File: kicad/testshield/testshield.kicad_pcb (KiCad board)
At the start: 2 copper layers, 26.7 x 55.9 mm, 6 parts, among them J1 ISP header, J2 Raspiheader, SW1 SW_Push, U1 ATMEGA328P-PU

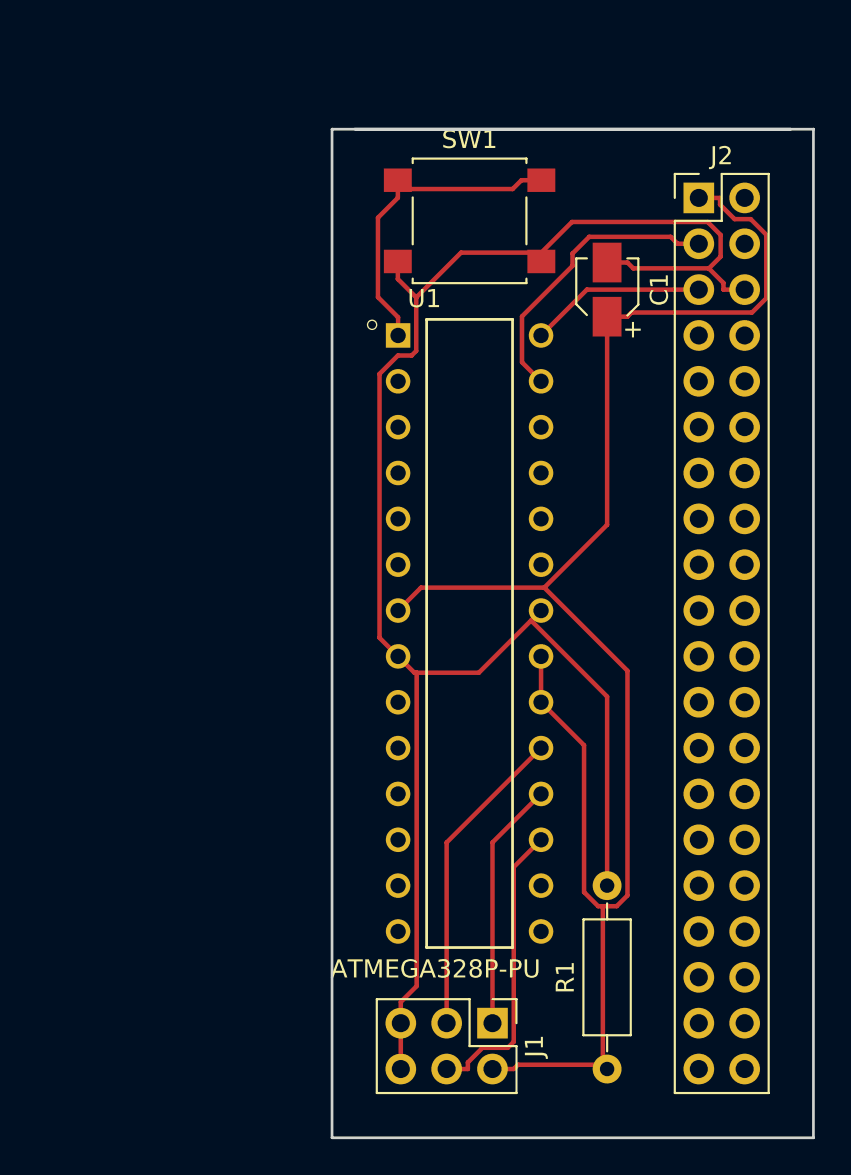
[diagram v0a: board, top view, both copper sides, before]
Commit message: update
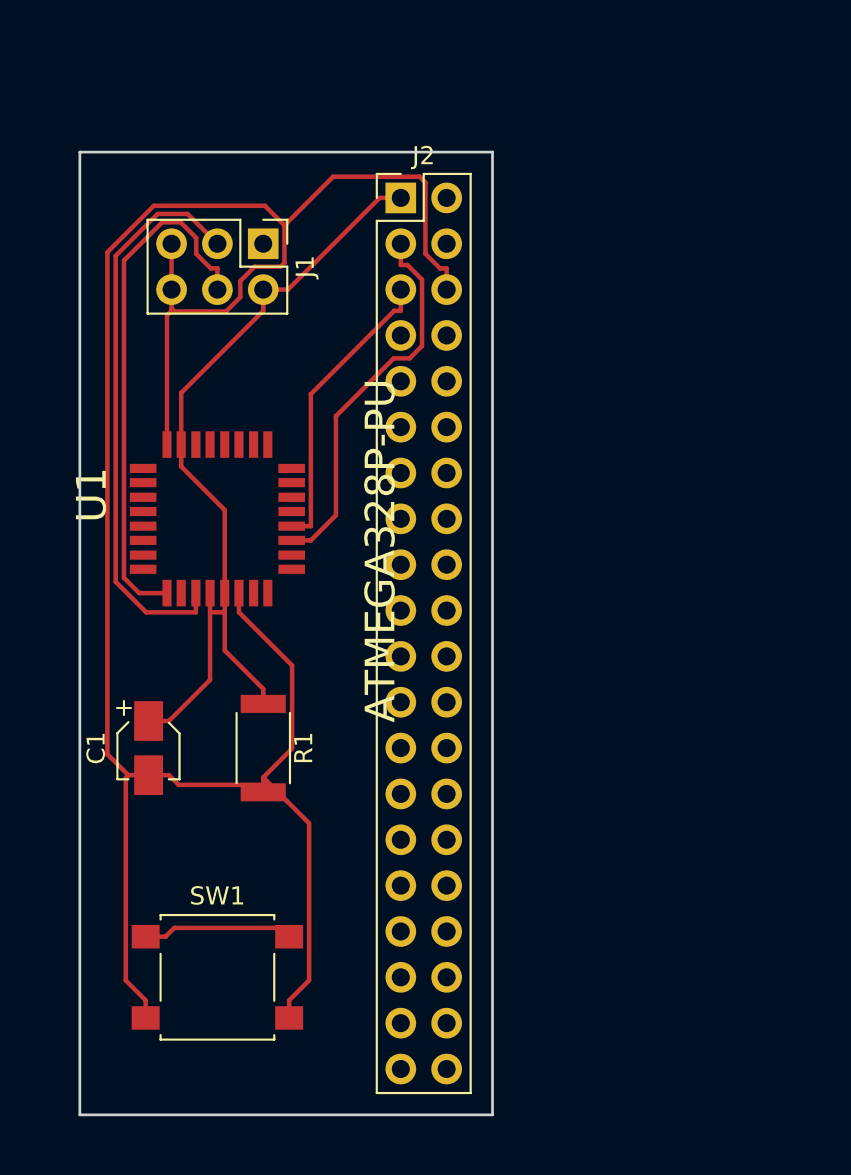
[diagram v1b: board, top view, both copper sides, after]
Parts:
- R1: footprint Resistors_THT:R_Axial_DIN0207_L6.3mm_D2.5mm_P10.16mm_Horizontal -> Resistors_SMD:R_2010
- U1: footprint ATMEGA328P-PU:DIP794W46P254L2967H457Q28B -> ATMEGA328P-AU:QFP80P900X900X120-32N
- moved J1 45.0 mm to (94.0, 87.6)
- moved SW1 44.2 mm to (91.4, 128.3)
- moved C1 35.9 mm to (87.6, 115.6), turned to 270 degrees
- moved R1 26.1 mm to (94.0, 115.6), turned to 270 degrees
- moved J2 16.5 mm to (101.6, 85.1)
- moved U1 15.3 mm to (91.4, 102.9), turned to 270 degrees
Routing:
- net +3V3: track 93.9 -> 46.4 mm
- net GNDD: track 102.5 -> 127.2 mm
- net Net-(J1-Pad3): track 17.4 -> 31.5 mm
- net Net-(J1-Pad1): track 13.8 -> 0.00 mm
- net Net-(J1-Pad4): track 16.4 -> 29.1 mm
- net Net-(SW1-Pad1): track 17.7 -> 8.64 mm
- net Net-(J2-Pad5): track 9.79 -> 16.4 mm
- net Net-(J2-Pad3): track 16.2 -> 21.3 mm
- added copper zone on F.Cu, net GNDD
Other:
- board size 26.7 x 55.9 mm -> 22.9 x 53.3 mm

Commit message: Add files via upload
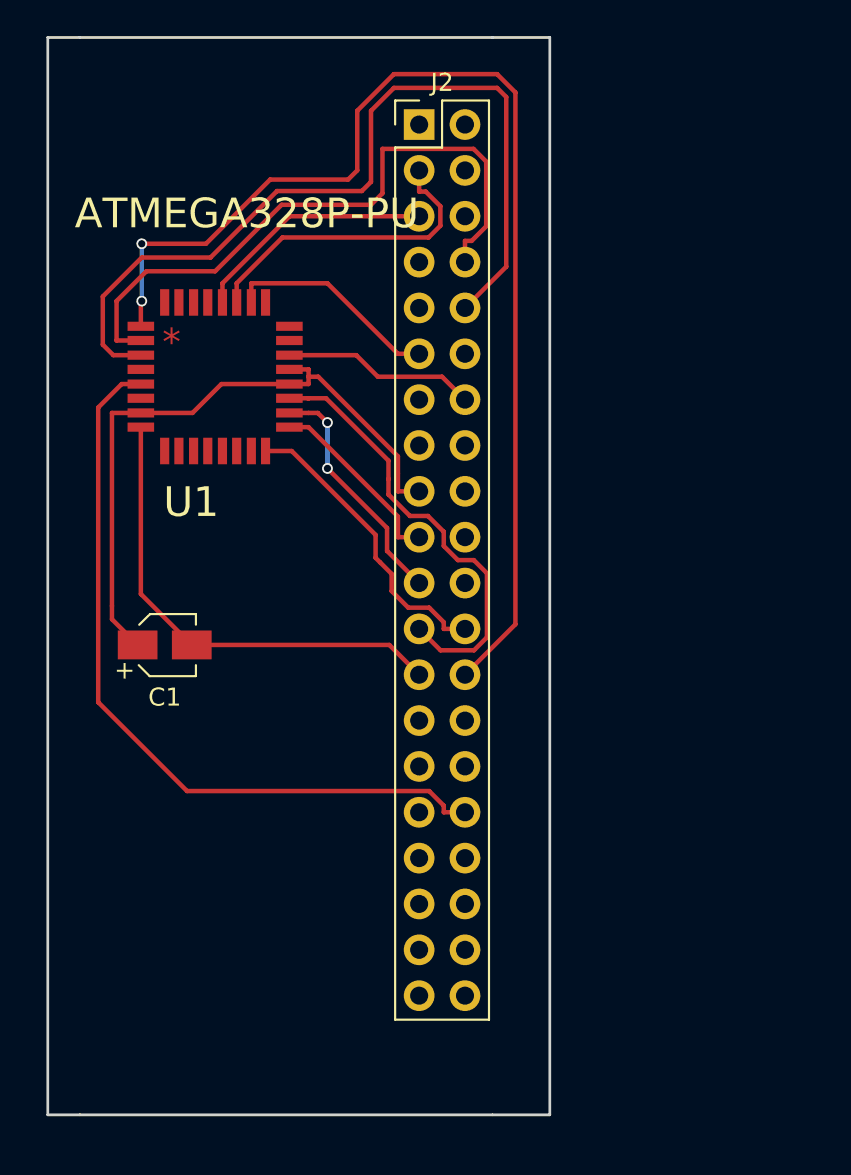
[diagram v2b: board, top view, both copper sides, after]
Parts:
- removed J1: ISP header, Pin_Headers:Pin_Header_Straight_2x03_Pitch2.54mm
- removed R1: 10k, Resistors_SMD:R_2010
- removed SW1: SW_Push, Buttons_Switches_SMD:SW_SPST_B3S-1000
- moved U1 7.88 mm to (91.3, 95.0), turned to 0 degrees
- moved C1 5.78 mm to (88.5, 109.9), turned to 0 degrees
- moved J2 4.19 mm to (102.6, 81.0)
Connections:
- J2 pad 1: +3V3 -> Net-(J2-Pad1)
- J2 pad 14: Net-(J2-Pad14) -> GNDD
- J2 pad 17: Net-(J2-Pad17) -> +3V3
- J2 pad 20: Net-(J2-Pad20) -> GNDD
- J2 pad 25: Net-(J2-Pad25) -> GNDD
- J2 pad 30: Net-(J2-Pad30) -> GNDD
- J2 pad 34: Net-(J2-Pad34) -> GNDD
- J2 pad 39: Net-(J2-Pad39) -> GNDD
- J2 pad 9: Net-(J2-Pad9) -> GNDD
- U1 pad 1: Net-(SW1-Pad1) -> Net-(J2-Pad26)
- U1 pad 16: Net-(U1-Pad16) -> Net-(J2-Pad24)
- U1 pad 17: Net-(J1-Pad4) -> Net-(J2-Pad19)
- U1 pad 18: Net-(J1-Pad1) -> Net-(J2-Pad21)
- U1 pad 19: Net-(J1-Pad3) -> Net-(J2-Pad23)
- U1 pad 2: Net-(U1-Pad2) -> Net-(J2-Pad8)
- U1 pad 26: Net-(U1-Pad26) -> Net-(J2-Pad11)
- U1 pad 3: Net-(U1-Pad3) -> Net-(J2-Pad10)
- U1 pad 5: Net-(U1-Pad5) -> Net-(J2-Pad32)
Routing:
- net GNDD: track 127.2 -> 37.3 mm
- net Net-(J2-Pad26): track 0.00 -> 65.0 mm, vias 0 -> 2
- net Net-(J2-Pad10): track 0.00 -> 47.3 mm
- net Net-(J2-Pad32): track 0.00 -> 42.3 mm
- net Net-(J2-Pad8): track 0.00 -> 35.5 mm
- net Net-(J1-Pad3): track 31.5 -> 0.00 mm
- net Net-(J1-Pad4): track 29.1 -> 0.00 mm
- net Net-(J2-Pad23): track 0.00 -> 24.7 mm
- net Net-(J2-Pad24): track 0.00 -> 16.6 mm
- net Net-(J2-Pad21): track 0.00 -> 13.3 mm, vias 0 -> 2
- net Net-(J2-Pad11): track 0.00 -> 12.0 mm
- net Net-(J2-Pad19): track 0.00 -> 10.4 mm
- net +3V3: track 46.4 -> 36.8 mm
- net Net-(SW1-Pad1): track 8.64 -> 0.00 mm
- net Net-(J2-Pad3): track 21.3 -> 17.4 mm
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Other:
- board size 22.9 x 53.3 mm -> 27.8 x 59.7 mm
- board text added: "*"
